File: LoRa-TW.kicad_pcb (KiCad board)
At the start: 4 copper layers, 12.4 x 24 mm, 38 parts, among them J1 MHF-I/U.FL, U1 SX1262IMLTRT, X1 TCXO, 32MHz, 2.0x1.6mm

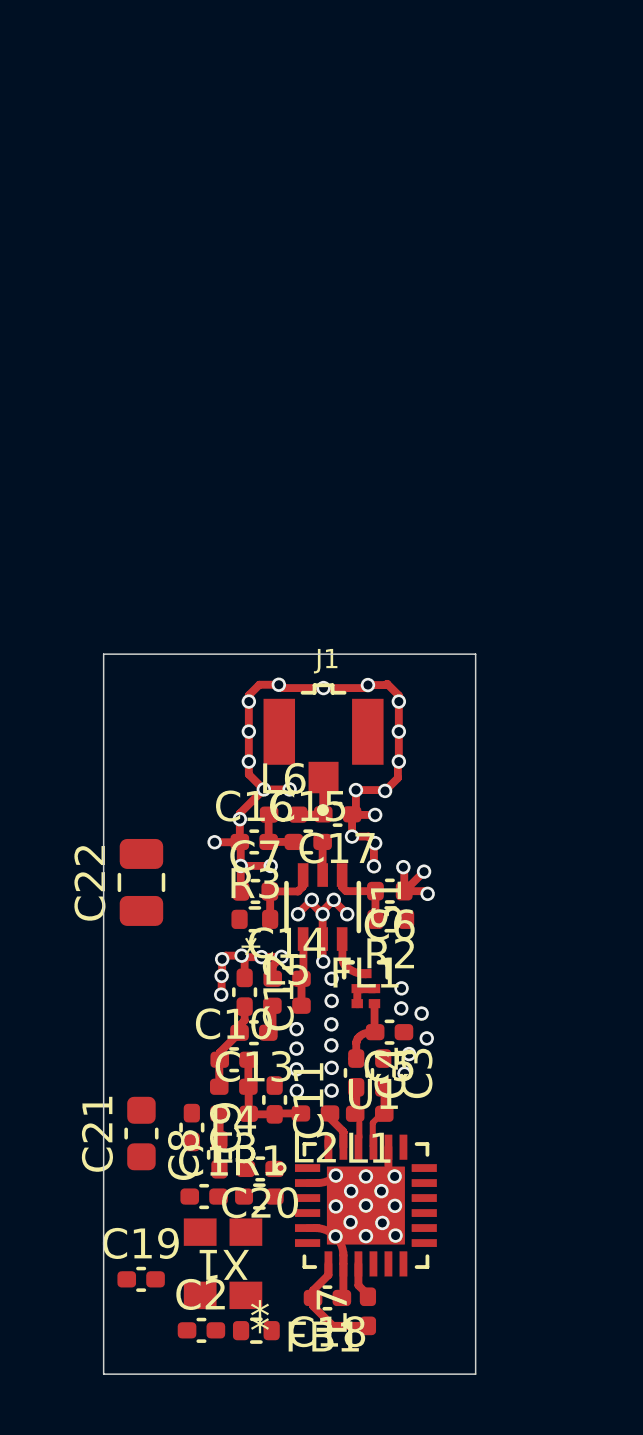
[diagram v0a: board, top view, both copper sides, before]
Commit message: update layout part
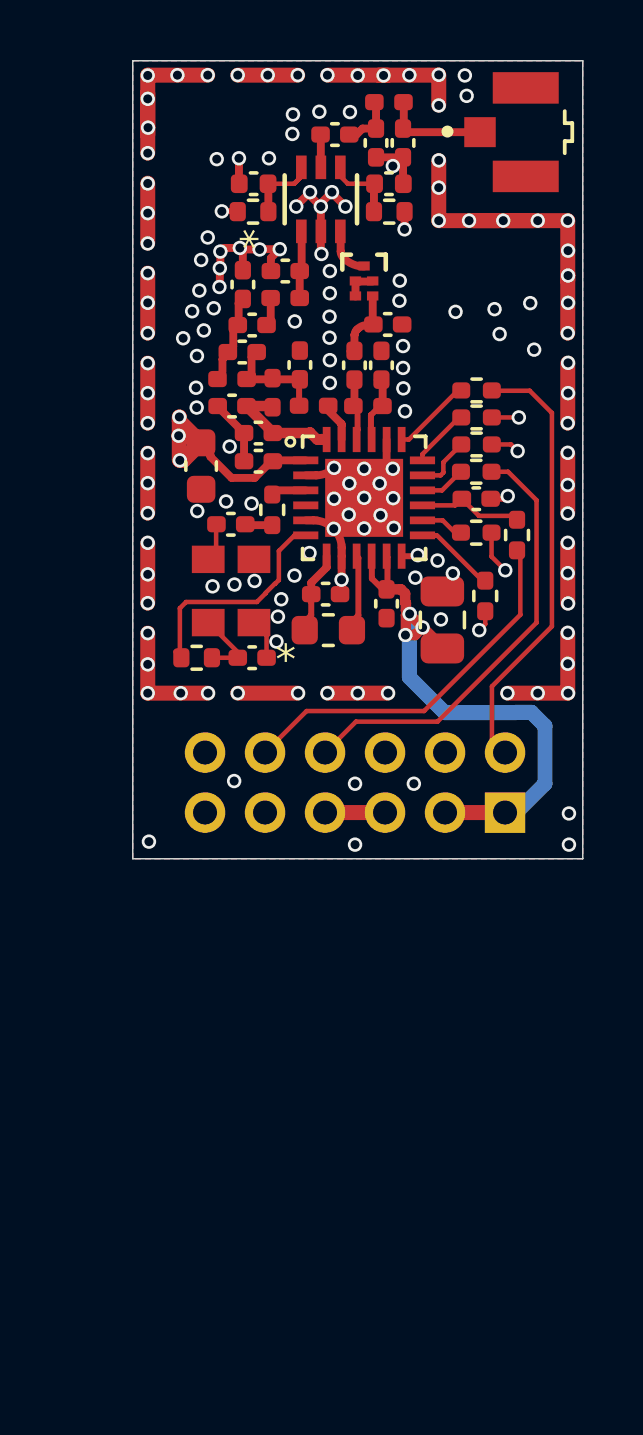
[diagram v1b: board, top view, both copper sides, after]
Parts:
- added C23: 100n, LoRa-TW:C_HF_0402_1005Metric, F.Cu at (158.5, 102.3)
- added J2: Conn_02x06_2.0mm, Connector_PinHeader_2.00mm:PinHeader_2x06_P2.00mm_Vertical, B.Cu at (159.5, 112.8)
- added J3: RFShield_OnePiece, LoRa-TW:ShieldCan, F.Cu at (154.6, 108.8)
- added R10: 33, LoRa-TW:R_HF_0402_1005Metric, F.Cu at (158.8, 105.5)
- added R4: 33, LoRa-TW:R_HF_0402_1005Metric, F.Cu at (158.5, 98.7)
- added R5: 33, LoRa-TW:R_HF_0402_1005Metric, F.Cu at (158.5, 99.6)
- added R6: 33, LoRa-TW:R_HF_0402_1005Metric, F.Cu at (158.5, 100.5)
- added R7: 33, LoRa-TW:R_HF_0402_1005Metric, F.Cu at (158.5, 101.4)
- added R8: 33, LoRa-TW:R_HF_0402_1005Metric, F.Cu at (159.9, 103.5)
- added R9: 33, LoRa-TW:R_HF_0402_1005Metric, F.Cu at (158.5, 103.4)
- L7: footprint LoRa-TW:L_HF_0402_1005Metric -> Inductor_SMD:L_0603_1608Metric
- moved C11 24.5 mm to (152.6, 97.8)
- moved C8 24.1 mm to (151.3, 100.1), turned to 0 degrees
- moved C9 24.1 mm to (150.4, 99.2), turned to 0 degrees
- moved L3 24.1 mm to (151.7, 98.8), turned to -90 degrees
- moved L6 24.0 mm to (155.6, 89.1)
- moved C19 24.0 mm to (155.5, 105.8), turned to -90 degrees
- moved C16 23.7 mm to (155.2, 90.4), turned to 90 degrees
- moved C15 23.6 mm to (153.8, 90.2), turned to 180 degrees
- moved C10 23.6 mm to (150.7, 97.4)
- moved C12 23.6 mm to (150.7, 95.2)
- moved C14 23.6 mm to (152.2, 94.7)
- moved C20 23.6 mm to (151.3, 101.0)
- moved C3 23.6 mm to (155.4, 97.8)
- moved C4 23.6 mm to (154.5, 97.8)
- moved C5 23.6 mm to (155.6, 96.5)
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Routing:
- net VDD: track 0.00 -> 50.9 mm, vias 0 -> 7
- net /MCU_ANT_{SW}: track 0.00 -> 22.6 mm, vias 0 -> 1
- net GND: track 41.5 -> 23.5 mm, vias 65 -> 152
- net Net-(J2-Pin_8): track 0.00 -> 14.8 mm
- net Net-(J2-Pin_2): track 0.00 -> 14.6 mm
- net Net-(J2-Pin_12): track 0.00 -> 14.1 mm, vias 0 -> 1
- net Net-(J2-Pin_4): track 0.00 -> 14.0 mm, vias 0 -> 1
- net Net-(J2-Pin_6): track 0.00 -> 13.2 mm, vias 0 -> 1
- net Net-(J2-Pin_10): track 0.00 -> 12.6 mm
- net /DIO2_ANT_{SW}: track 0.00 -> 12.4 mm, vias 0 -> 2
- net Net-(J2-Pin_9): track 0.00 -> 10.9 mm, vias 0 -> 1
- net /DIO3_CLK_{EN}: track 0.00 -> 7.73 mm
- net /~{RESET}: track 0.00 -> 3.53 mm
- net /DIO1_INT: track 0.00 -> 3.15 mm
- net Net-(U1-VR_PA): track 1.13 -> 3.94 mm
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- added copper zone on B.Cu, net GND
- added copper zone on F.Cu, net GND
- added copper zone on In1.Cu, net GND
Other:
- board size 12.4 x 24 mm -> 15 x 26.6 mm
